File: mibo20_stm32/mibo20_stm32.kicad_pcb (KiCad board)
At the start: 2 copper layers, 33 x 17.8 mm, 24 parts, among them J1 Conn_01x02, J2 Conn_01x13, J3 Conn_01x13, J4 USB_B_Micro, J5 Conn_01x04, SW1 Reset, U1 STM32F070F6Px, U2 AMS1117-3.3, Y1 8MHz

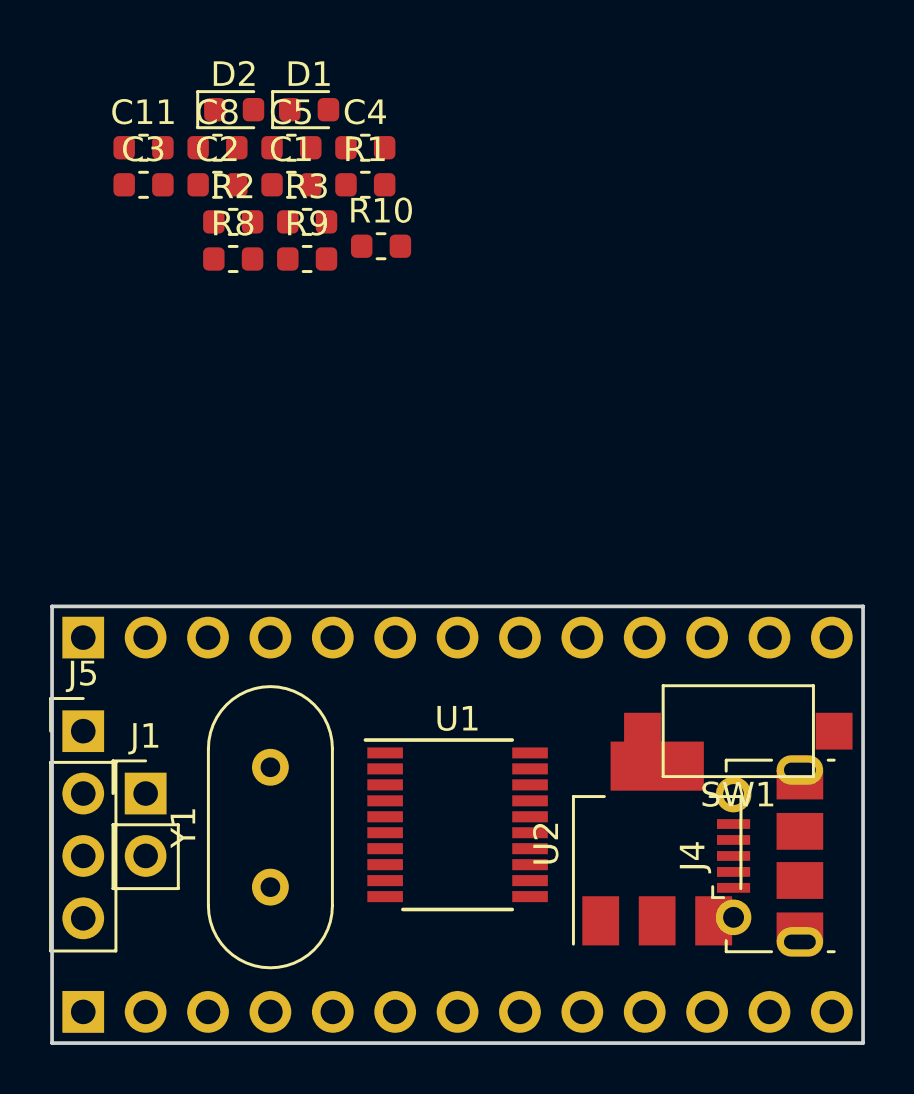
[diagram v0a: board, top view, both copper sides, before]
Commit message: V1.0 - Fully routed with description
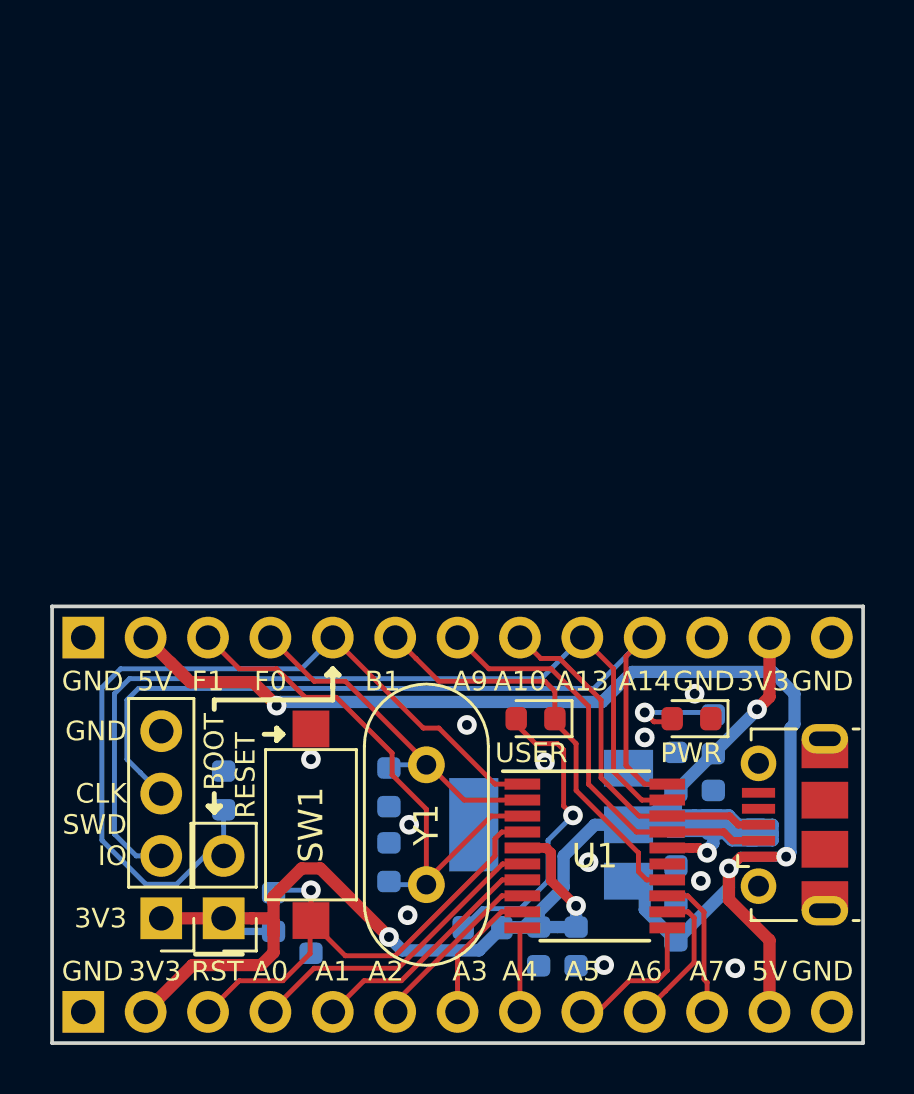
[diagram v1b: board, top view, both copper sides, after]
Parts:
- removed C11: 4.7uF, Capacitor_SMD:C_0603_1608Metric
- removed R10: 1k, Resistor_SMD:R_0603_1608Metric
- removed R8, R9: 22R, Resistor_SMD:R_0603_1608Metric
- added C6: 10nF, Capacitor_SMD:C_0603_1608Metric, B.Cu at (157.2, 101.5)
- added C7: 1uF, Capacitor_SMD:C_0603_1608Metric, B.Cu at (155.7, 101.5)
- added C9: 4.7uF, Capacitor_SMD:C_0603_1608Metric, B.Cu at (161.3, 94.4)
- added R4: 1k, Resistor_SMD:R_0603_1608Metric, B.Cu at (162.8, 92.8)
- C1, C2, C5, C8, R1, R2, R3, U2: moved to B.Cu
- C3: value 10nF -> 100nF; moved to B.Cu
- C4: value 100nF -> 4.7uF; moved to B.Cu
- D2: value GREEN -> RED
- U1: value STM32F070F6Px -> STM32x0xxFxPx
- moved C8 36.6 mm to (161.3, 100.5), turned to 90 degrees
- moved C5 32.0 mm to (162.8, 95.9), turned to 90 degrees
- moved C3 31.3 mm to (146.4, 101.0), turned to 270 degrees
- moved C4 31.1 mm to (161.3, 97.4), turned to 270 degrees
- moved D2 31.0 mm to (161.9, 92.2), turned to 180 degrees
- moved R3 29.6 mm to (153.4, 100.7)
- moved C2 28.4 mm to (149.6, 98.0), turned to 90 degrees
- moved R2 28.1 mm to (144.9, 100.1), turned to 270 degrees
- moved D1 26.5 mm to (155.6, 92.2), turned to 180 degrees
- moved R1 25.3 mm to (142.9, 95.1), turned to 90 degrees
- moved C1 24.9 mm to (149.6, 95.0), turned to 270 degrees
- moved SW1 17.8 mm to (146.4, 96.5), turned to 90 degrees
- moved J5 8.26 mm to (140.3, 100.3), turned to 180 degrees
- moved Y1 8.07 mm to (151.1, 94.1), turned to 270 degrees
- moved J1 5.99 mm to (142.9, 100.3), turned to 180 degrees
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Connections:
- D1 pad 1: Net-(D1-Pad1) -> /LED1
- D1 pad 2: +3V3 -> Net-(D1-Pad2)
- D2 pad 1: Net-(D2-Pad1) -> GND
- D2 pad 2: +3V3 -> Net-(D2-Pad2)
- J1 pad 1: /BOOT0 -> +3V3
- J1 pad 2: +3V3 -> /BOOT0
- J2 pad 10: /SWDCLK -> /PA6
- J2 pad 11: GND -> /PA7
- J2 pad 4: /OSC_IN -> /PA0
- J2 pad 5: /OSC_OUT -> /PA1
- J2 pad 6: /LED1 -> /PA2
- J2 pad 7: /PA6 -> /PA3
- J2 pad 8: /PA7 -> /PA4
- J2 pad 9: /SWDIO -> /PA5
- J3 pad 10: /PA10 -> /PA14
- J3 pad 11: /PA11 -> GND
- J3 pad 3: /BOOT0 -> /OSC_OUT
- J3 pad 4: /PA0 -> /OSC_IN
- J3 pad 5: /PA1 -> /BOOT0
- J3 pad 6: /PA2 -> /LED1
- J3 pad 7: /PA3 -> /PA11
- J3 pad 8: /PA4 -> /PA10
- J3 pad 9: /PA5 -> /PA13
- J4 pad 4: Net-(J4-Pad4) -> (no net)
- J5 pad 2: /SWDIO -> /PA13
- J5 pad 3: /SWDCLK -> /PA14
- R3 pad 1: /LED1 -> Net-(D1-Pad2)
- R3 pad 2: Net-(D1-Pad1) -> +3V3
- U1 pad 19: /SWDIO -> /PA13
- U1 pad 20: /SWDCLK -> /PA14
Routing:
- net +3V3: track 0.00 -> 74.4 mm, vias 0 -> 4
- net /5V: track 0.00 -> 54.4 mm, vias 0 -> 3
- net /PA13: track 0.00 -> 36.6 mm
- net /BOOT0: track 0.00 -> 34.7 mm
- net /PA14: track 0.00 -> 34.0 mm
- net /OSC_OUT: track 0.00 -> 22.4 mm
- net /RESET: track 0.00 -> 22.1 mm, vias 0 -> 1
- net /PA11: track 0.00 -> 17.5 mm
- net /LED1: track 0.00 -> 17.5 mm
- net /PA10: track 0.00 -> 14.7 mm
- net /OSC_IN: track 0.00 -> 14.7 mm
- net /PA0: track 0.00 -> 12.8 mm
- net Net-(D1-Pad2): track 0.00 -> 12.6 mm, vias 0 -> 1
- net /PA1: track 0.00 -> 9.94 mm
- net /PA2: track 0.00 -> 7.36 mm
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- added copper zone on B.Cu, net GND
- added copper zone on F.Cu, net GND
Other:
- net class Default: trace_width 0.25 -> 0.2
- net class Power added: clearance 0.2, trace_width 0.5, via_dia 0.8, via_drill 0.4
- net class USB added: clearance 0.2, trace_width 0.3, via_dia 0.8, via_drill 0.4
- board text added: "3V3"
- board text added: "5V"
- board text added: "A0"
- board text added: "A1"
- board text added: "A10"
- board text added: "A13"
- board text added: "A14"
- board text added: "A2"
- board text added: "A3"
- board text added: "A4"
- board text added: "A5"
- board text added: "A6"
- board text added: "A7"
- board text added: "A9"
- board text added: "B1"
- board text added: "BOOT"
- board text added: "CLK"
- board text added: "F0"
- board text added: "F1"
- board text added: "GND"
- board text added: "IO"
- board text added: "MIBO20 STM32"
- board text added: "PWR"
- board text added: "RESET"
- board text added: "RST"
- board text added: "SWD"
- board text added: "USER"

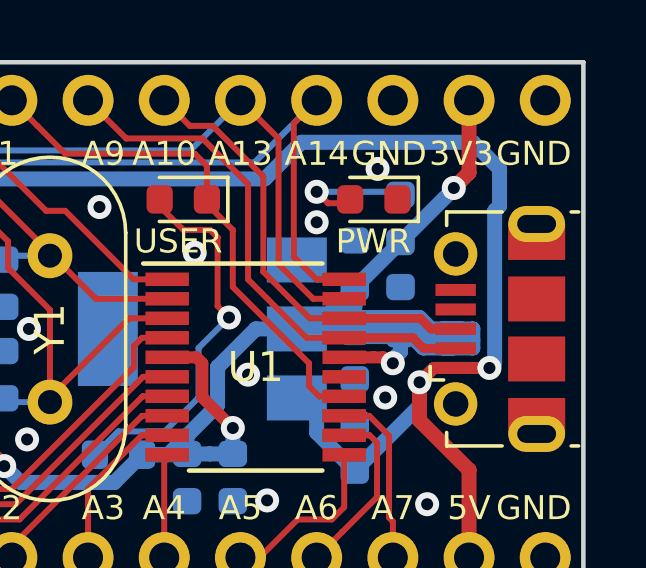
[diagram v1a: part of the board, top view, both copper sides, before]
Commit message: small trace tweak
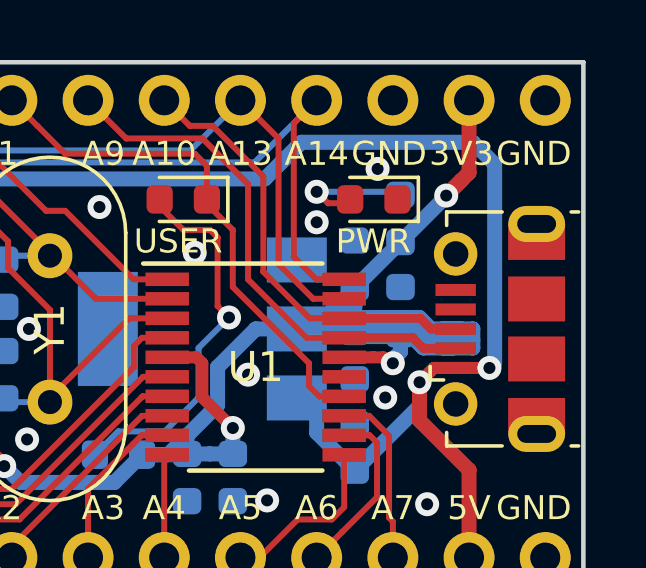
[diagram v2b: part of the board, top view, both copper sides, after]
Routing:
- net +3V3: track 74.4 -> 75.0 mm
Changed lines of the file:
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@@
     (thickness 1.6)
     (drawings 55)
-    (tracks 274)
+    (tracks 275)
     (zones 0)
     (modules 24)
@@
   (segment (start 162.433 96.774) (end 161.417 96.774) (width 0.5) (layer B.Cu) (net 5))
   (segment (start 165.227 96.52) (end 164.211 96.52) (width 0.5) (layer B.Cu) (net 5))
-  (via (at 164.592 91.821) (size 0.8) (drill 0.4) (layers F.Cu B.Cu) (net 5))
+  (via (at 164.338 92.075) (size 0.8) (drill 0.4) (layers F.Cu B.Cu) (net 5))
   (segment (start 161.912 97.465) (end 160.938 97.465) (width 0.4) (layer F.Cu) (net 5))
   (via (at 149.606 101.092) (size 0.8) (drill 0.4) (layers F.Cu B.Cu) (net 5))
@@
   (segment (start 154.686 100.711) (end 155.6765 100.711) (width 0.5) (layer B.Cu) (net 5))
   (segment (start 162.814 93.6245) (end 162.761772 93.6245) (width 0.5) (layer B.Cu) (net 5))
-  (segment (start 164.465 91.9735) (end 162.814 93.6245) (width 0.5) (layer B.Cu) (net 5))
-  (segment (start 165.1 91.313) (end 164.592 91.821) (width 0.5) (layer F.Cu) (net 5))
-  (segment (start 165.1 88.9) (end 165.1 91.313) (width 0.5) (layer F.Cu) (net 5))
   (segment (start 161.29 96.6215) (end 162.763 96.6215) (width 0.5) (layer B.Cu) (net 5))
   (segment (start 165.227 97.155) (end 164.211 97.155) (width 0.5) (layer B.Cu) (net 5))
   (segment (start 163.449 96.139) (end 163.716018 96.406018) (width 0.5) (layer B.Cu) (net 5))
+  (segment (start 165.1 88.9) (end 165.1 91.313) (width 0.5) (layer F.Cu) (net 5))
+  (segment (start 164.846 91.567) (end 164.338 92.075) (width 0.5) (layer F.Cu) (net 5))
+  (segment (start 164.846 91.567) (end 164.592 91.821) (width 0.5) (layer F.Cu) (net 5))
+  (segment (start 165.1 91.313) (end 164.846 91.567) (width 0.5) (layer F.Cu) (net 5))
+  (segment (start 164.338 92.1005) (end 162.814 93.6245) (width 0.5) (layer B.Cu) (net 5))
+  (segment (start 164.338 92.075) (end 164.338 92.1005) (width 0.5) (layer B.Cu) (net 5))
   (segment (start 163.926999 97.820001) (end 165.779999 97.820001) (width 0.4) (layer B.Cu) (net 6))
   (segment (start 163.449 98.298) (end 163.926999 97.820001) (width 0.4) (layer B.Cu) (net 6))
@@
   (segment (start 160.02 99.9745) (end 161.29 101.2445) (width 0.5) (layer B.Cu) (net 6))
   (segment (start 160.02 99.06) (end 160.02 99.9745) (width 0.5) (layer B.Cu) (net 6))
-  (segment (start 145.184 91.520032) (end 145.034 91.670032) (width 0.5) (layer B.Cu) (net 6))
-  (segment (start 158.288968 91.520032) (end 145.184 91.520032) (width 0.5) (layer B.Cu) (net 6))
-  (segment (start 159.512 90.297) (end 158.288968 91.520032) (width 0.5) (layer B.Cu) (net 6))
-  (segment (start 165.95349 97.64651) (end 165.95349 92.585072) (width 0.5) (layer B.Cu) (net 6))
-  (segment (start 165.8 97.8) (end 165.95349 97.64651) (width 0.5) (layer B.Cu) (net 6))
-  (segment (start 166.116 92.422562) (end 166.116 91.186) (width 0.5) (layer B.Cu) (net 6))
-  (segment (start 166.116 91.186) (end 165.227 90.297) (width 0.5) (layer B.Cu) (net 6))
-  (segment (start 165.95349 92.585072) (end 166.116 92.422562) (width 0.5) (layer B.Cu) (net 6))
-  (segment (start 165.227 90.297) (end 159.512 90.297) (width 0.5) (layer B.Cu) (net 6))
   (segment (start 163.449 98.298) (end 163.449 99.568) (width 0.5) (layer F.Cu) (net 6))
   (segment (start 163.449 99.568) (end 165.100001 101.219001) (width 0.5) (layer F.Cu) (net 6))
   (segment (start 165.100001 104.14) (end 165.100001 101.219001) (width 0.5) (layer F.Cu) (net 6))
+  (segment (start 145.184 91.520032) (end 145.034 91.670032) (width 0.5) (layer B.Cu) (net 6))
+  (segment (start 165.95349 97.64651) (end 165.95349 91.02349) (width 0.5) (layer B.Cu) (net 6))
+  (segment (start 165.8 97.8) (end 165.95349 97.64651) (width 0.5) (layer B.Cu) (net 6))
+  (segment (start 165.227 90.297) (end 159.512 90.297) (width 0.5) (layer B.Cu) (net 6))
+  (segment (start 159.512 90.297) (end 158.288968 91.520032) (width 0.5) (layer B.Cu) (net 6))
+  (segment (start 165.95349 91.02349) (end 165.227 90.297) (width 0.5) (layer B.Cu) (net 6))
+  (segment (start 158.288968 91.520032) (end 145.184 91.520032) (width 0.5) (layer B.Cu) (net 6))
   (segment (start 142.875 97.79) (end 142.875 96.5455) (width 0.2) (layer B.Cu) (net 7))
   (segment (start 142.113 97.79) (end 142.875 97.79) (width 0.2) (layer B.Cu) (net 7))
